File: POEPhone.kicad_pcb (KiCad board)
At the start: 2 copper layers, 1 part, among them U1 ESP-07S

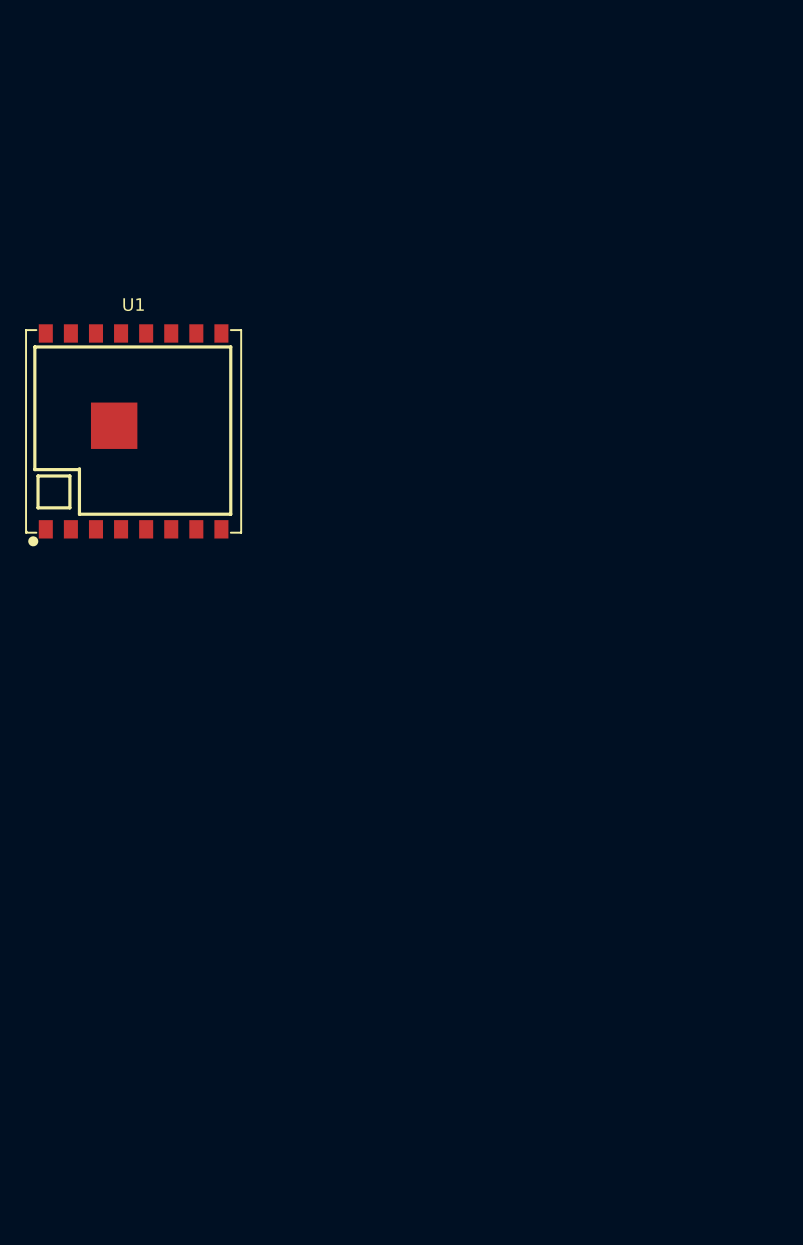
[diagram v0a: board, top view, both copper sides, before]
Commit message: Rough initial layout
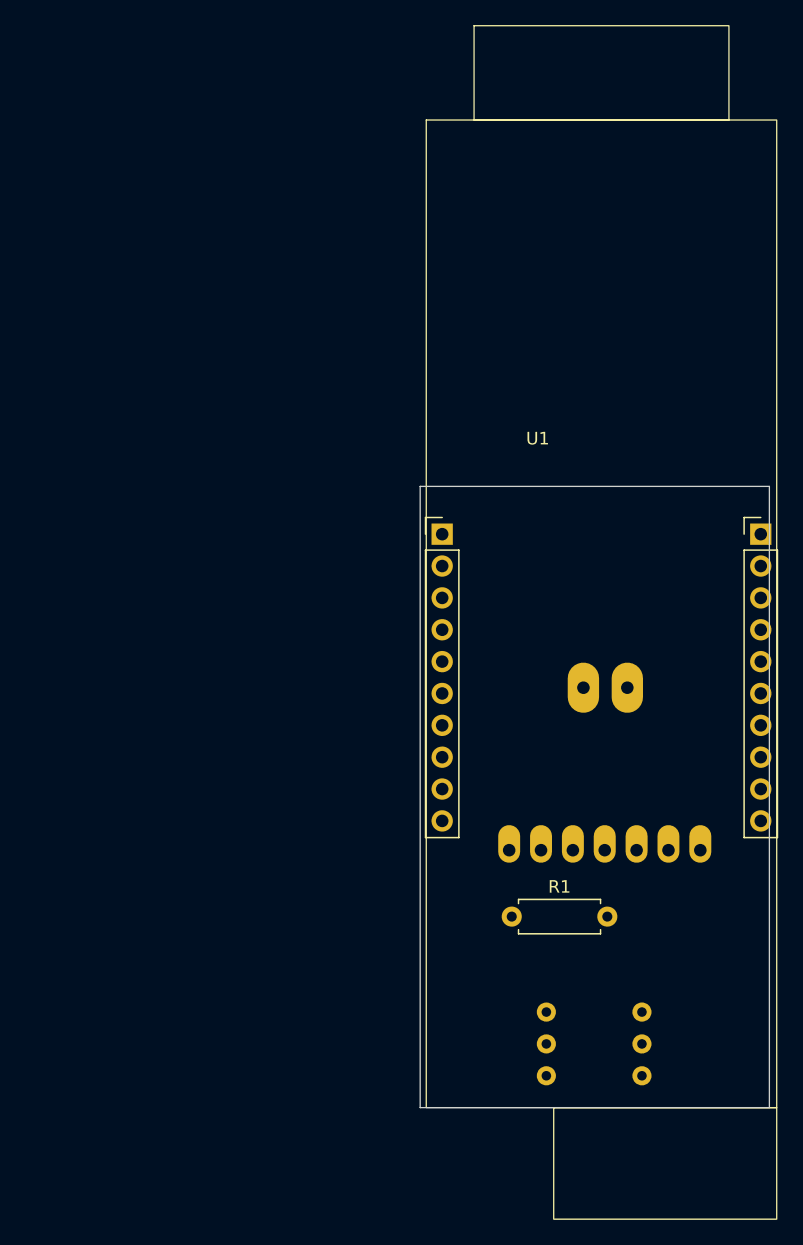
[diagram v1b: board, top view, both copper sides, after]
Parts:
- added R1: 100k, Resistor_THT:R_Axial_DIN0207_L6.3mm_D2.5mm_P7.62mm_Horizontal, F.Cu at (135.7, 91.4)
- added U2: mems-mic, mems-mic:mems-mic-round, B.Cu at (142.2, 101.6)
- added U3: adafruit-MAX98357, adafruit-MAX98357:adafruit-MAX98357, B.Cu at (143.0, 79.2)
- U1: value ESP-07S -> ~; footprint jlc_footprints:WIRELM-SMD_ESP-07S -> molex-poe:molex-poe
- moved U1 41.6 mm to (142.8, 71.1)
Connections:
- U1 pad 12: unconnected-(U1-IO0-Pad12) -> I2S_MIC_DATA
- U1 pad 2: unconnected-(U1-ADC-Pad2) -> +3V3
- U1 pad 3: unconnected-(U1-EN-Pad3) -> GND
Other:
- board outline added: 27.8 x 49.5 mm
